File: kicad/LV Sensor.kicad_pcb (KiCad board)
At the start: 2 copper layers, 79.2 x 47 mm, 73 parts, among them IC1 MCP2517FDT-H_SL, IC2 L78L05ABUTR, IC3 TLV74133PDBVR, IC4 TLV74125PDBVR, IC5 MSPM0C1104SDGS20R, J1 Screw_Terminal_01x02, J16 USB_B_Micro, J2 Screw_Terminal_01x02, J3 Screw_Terminal_01x02, J4 Screw_Terminal_01x02, J5 Screw_Terminal_01x02, J6 43650-0401, SW1 SW_Push, U0 AP63205WU-7, U10 MCP3204-CI/P, U3 FT231XS-R, U6 DSC1001DL5-020.0000T, U7 ADS114S06BIPBSR, U8 LM2662MX/NOPB, U9 ATA6561-GAQW-N

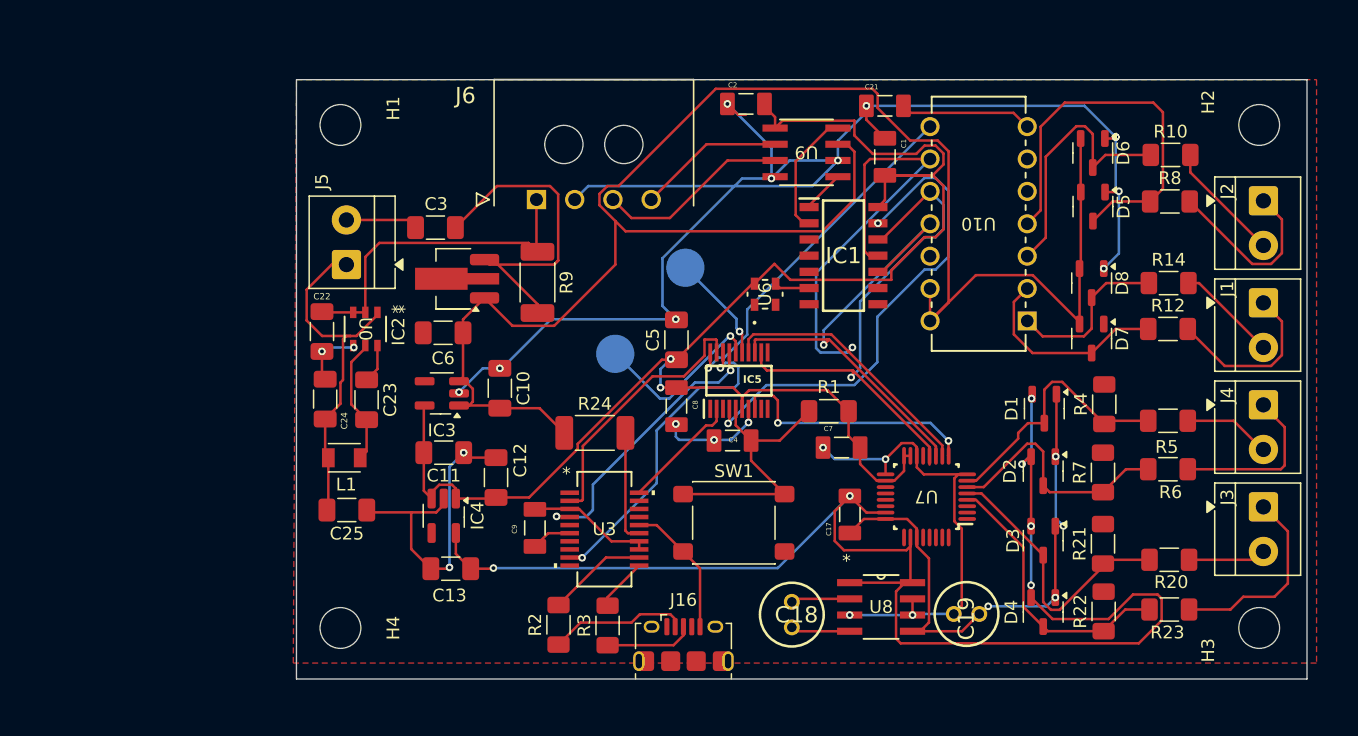
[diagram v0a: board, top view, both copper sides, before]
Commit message: finished v1
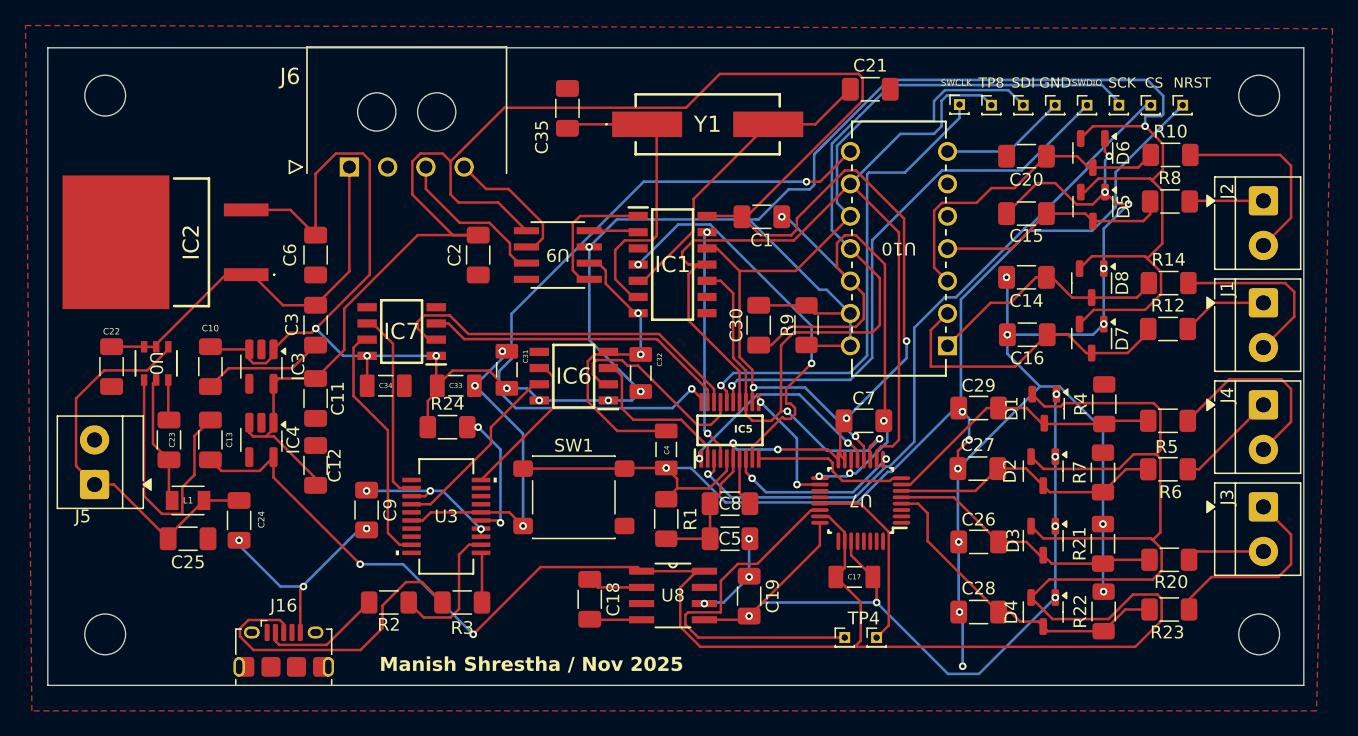
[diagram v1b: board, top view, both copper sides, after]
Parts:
- removed U6: DSC1001DL5-020.0000T, LV-Sensor-Footprints-Lib:CDFN4_2P5X2_MCH
- added C14: 0.1uF, Capacitor_SMD:C_1206_3216Metric_Pad1.33x1.80mm_HandSolder, F.Cu at (206.8, 67.8)
- added C15: 0.1uF, Capacitor_SMD:C_1206_3216Metric_Pad1.33x1.80mm_HandSolder, F.Cu at (206.8, 62.8)
- added C16: 0.1uF, Capacitor_SMD:C_1206_3216Metric_Pad1.33x1.80mm_HandSolder, F.Cu at (206.8, 72.2)
- added C20: 0.1uF, Capacitor_SMD:C_1206_3216Metric_Pad1.33x1.80mm_HandSolder, F.Cu at (206.8, 58.2)
- added C26: 0.1uF, Capacitor_SMD:C_1206_3216Metric_Pad1.33x1.80mm_HandSolder, F.Cu at (203.0, 88.5)
- added C27: 0.1uF, Capacitor_SMD:C_1206_3216Metric_Pad1.33x1.80mm_HandSolder, F.Cu at (202.9, 82.8)
- added C28: 0.1uF, Capacitor_SMD:C_1206_3216Metric_Pad1.33x1.80mm_HandSolder, F.Cu at (203.0, 94.0)
- added C29: 0.1uF, Capacitor_SMD:C_1206_3216Metric_Pad1.33x1.80mm_HandSolder, F.Cu at (203.0, 78.0)
- added C30: 0.1uF, Capacitor_SMD:C_1206_3216Metric_Pad1.33x1.80mm_HandSolder, F.Cu at (185.8, 71.5)
- added C31: 0.01uF, ADC2_AND_4:CAPC3216X140N, F.Cu at (166.0, 75.0)
- added C32: 0.01uF, ADC2_AND_4:CAPC3216X140N, F.Cu at (176.5, 75.2)
- added C33: 0.01uF, ADC2_AND_4:CAPC3216X140N, F.Cu at (162.0, 76.2)
- added C34: 0.01uF, ADC2_AND_4:CAPC3216X140N, F.Cu at (156.5, 76.2)
- added C35: 47pF, Capacitor_SMD:C_1206_3216Metric_Pad1.33x1.80mm_HandSolder, F.Cu at (170.8, 54.5)
- added IC6: ISO6721BDR, LV-Sensor-Footprints-Lib:SOIC127P600X175-8N, F.Cu at (171.2, 75.5)
- added IC7: ISO6721BDR, LV-Sensor-Footprints-Lib:SOIC127P600X175-8N, F.Cu at (157.8, 72.0)
- added TP10: TestPoint, Connector_PinHeader_1.00mm:PinHeader_1x01_P1.00mm_Vertical, F.Cu at (214.0, 54.2)
- added TP3: TestPoint, Connector_PinHeader_1.00mm:PinHeader_1x01_P1.00mm_Vertical, F.Cu at (192.5, 96.0)
- added TP4: TestPoint, Connector_PinHeader_1.00mm:PinHeader_1x01_P1.00mm_Vertical, F.Cu at (195.0, 96.0)
- added TP5: TestPoint, Connector_PinHeader_1.00mm:PinHeader_1x01_P1.00mm_Vertical, F.Cu at (209.0, 54.2)
- added TP6: TestPoint, Connector_PinHeader_1.00mm:PinHeader_1x01_P1.00mm_Vertical, F.Cu at (219.0, 54.2)
- added TP7: TestPoint, Connector_PinHeader_1.00mm:PinHeader_1x01_P1.00mm_Vertical, F.Cu at (216.5, 54.2)
- added TP8: TestPoint, Connector_PinHeader_1.00mm:PinHeader_1x01_P1.00mm_Vertical, F.Cu at (204.0, 54.2)
- added TP9: TestPoint, Connector_PinHeader_1.00mm:PinHeader_1x01_P1.00mm_Vertical, F.Cu at (206.5, 54.2)
- added Y1: 830017146, LV-Sensor-Footprints-Lib:830017146, F.Cu at (181.8, 55.8)
- C1, C2, C7: value 0.1µF -> 0.1uF; footprint ADC2_AND_4:CAPC3216X125N -> Capacitor_SMD:C_1206_3216Metric_Pad1.33x1.80mm_HandSolder
- C18, C19: footprint ADC2_AND_4:A750_5X7_ -> Capacitor_SMD:C_1206_3216Metric_Pad1.33x1.80mm_HandSolder
- C21: value 0.01µf -> 47pF; footprint ADC2_AND_4:CAPC3216X140N -> Capacitor_SMD:C_1206_3216Metric_Pad1.33x1.80mm_HandSolder
- C23: value 100nF -> 0.1uF
- C4: value 0.01 µF -> 0.01 uF
- C5: value 10u -> 10uF
- C8: value 100n -> 0.1uF; footprint ADC2_AND_4:CAPC3216X125N -> Capacitor_SMD:C_1206_3216Metric_Pad1.33x1.80mm_HandSolder
- C9: value 100nF -> 0.1uF; footprint ADC2_AND_4:CAPC3216X125N -> Capacitor_SMD:C_1206_3216Metric_Pad1.33x1.80mm_HandSolder
- IC2: value L78L05ABUTR -> MC7805CD2TR4G; footprint Package_TO_SOT_SMD:SOT-89-3_Handsoldering -> LV-Sensor-Footprints-Lib:MC7805CD2TR4G
- R24: footprint Resistor_SMD:R_2010_5025Metric_Pad1.40x2.65mm_HandSolder -> Resistor_SMD:R_1206_3216Metric_Pad1.30x1.75mm_HandSolder
- R9: value 1k -> 20k; footprint Resistor_SMD:R_2010_5025Metric_Pad1.40x2.65mm_HandSolder -> Resistor_SMD:R_1206_3216Metric_Pad1.30x1.75mm_HandSolder
- TP1, TP2: footprint TestPoint:TestPoint_Pad_D3.0mm -> Connector_PinHeader_1.00mm:PinHeader_1x01_P1.00mm_Vertical; moved to F.Cu
- moved TP2 34.0 mm to (211.5, 54.2), turned to 0 degrees
- moved TP1 33.3 mm to (201.5, 54.2), turned to 0 degrees
- moved J16 31.4 mm to (148.5, 97.0)
- moved J5 26.2 mm to (133.7, 84.0)
- moved C2 24.1 mm to (163.8, 66.0), turned to 90 degrees
- moved C10 22.8 mm to (142.8, 74.8), turned to 90 degrees
- moved IC2 22.5 mm to (139.5, 65.0), turned to 90 degrees
- moved C13 21.4 mm to (142.8, 80.5), turned to 90 degrees
- moved R9 21.4 mm to (189.5, 71.5)
- moved U9 21.1 mm to (170.0, 66.0)
- moved H1 18.6 mm to (134.5, 53.5)
- moved H4 18.5 mm to (134.5, 95.8)
- moved C19 17.1 mm to (185.0, 92.8), turned to -90 degrees
- moved C22 16.7 mm to (135.0, 74.8)
- moved U0 16.6 mm to (138.5, 74.5)
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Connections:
- net Net-(IC1-SCK) renamed SCK
- net Net-(IC1-SDI) renamed SDO
- net Net-(IC1-SDO) renamed SDI
- net Net-(IC5-PA1_/_NRST) renamed NRST
- C19 pad 1: -2V5 -> GND
- C19 pad 2: GND -> -2V5
- C21 pad 1: GND -> Net-(IC1-OSC2)
- C21 pad 2: Net-(U10-DGND) -> GND
- C3 pad 2: Net-(IC2-VIN) -> +12V
- C6 pad 1: GND -> +5V
- C6 pad 2: +5V -> GND
- IC1 pad 4: unconnected-(IC1-~{INT}-Pad4) -> CAN_FD_INT
- IC1 pad 5: unconnected-(IC1-OSC2-Pad5) -> Net-(IC1-OSC2)
- IC2 pad 1: +5V -> +12V
- IC2 pad 3: Net-(IC2-VIN) -> +5V
- IC5 pad 1: unconnected-(IC5-PA26_/_A1-Pad1) -> ADC_DRDY
- IC5 pad 10: unconnected-(IC5-PA6-Pad10) -> ADC_START
- IC5 pad 11: unconnected-(IC5-PA11-Pad11) -> ADC_RESET
- IC5 pad 3: unconnected-(IC5-PA28_/_A5-Pad3) -> EXTERNAL_CS
- IC5 pad 9: unconnected-(IC5-PA4-Pad9) -> CAN_FD_INT
- R9 pad 1: +12V -> +5V
- R9 pad 2: Net-(IC2-VIN) -> +5V
- U10 pad 7: Net-(U10-DGND) -> GND
- U3 pad 2: UART0_RTS -> UART0_RTS_ISOLA
- U3 pad 20: UART0_TX -> UART0_TX_ISOLA
- U3 pad 4: UART0_RX -> UART0_RX_ISOLA
- U3 pad 9: UART0_CTS -> UART0_CTS_ISOLA
- U7 pad 13: unconnected-(U7-DRDY_N-Pad13) -> ADC_DRDY
- U7 pad 18: +3V3 -> ADC_RESET
- U7 pad 21: unconnected-(U7-GPIO1-Pad21) -> Net-(U7-GPIO1)
- U7 pad 22: unconnected-(U7-GPIO0-Pad22) -> Net-(U7-GPIO0)
- U7 pad 8: GND -> ADC_START
- U8 pad 7: GND -> unconnected-(U8-OSC-Pad7)
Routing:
- net +5V: track 144.0 -> 213.0 mm, vias 0 -> 9
- net +2V5: track 116.4 -> 175.7 mm, vias 6 -> 2
- net NRST: track 21.7 -> 80.7 mm, vias 0 -> 1
- net EXTERNAL_CS: track 0.00 -> 55.9 mm, vias 0 -> 1
- net GND: track 212.0 -> 262.6 mm, vias 22 -> 30
- net SCK: track 38.6 -> 81.8 mm, vias 1 -> 2
- net +3V3: track 126.5 -> 169.7 mm, vias 2 -> 4
- net Net-(IC5-PA19_/_SWDIO): track 8.48 -> 43.7 mm
- net CAN_FD_INT: track 0.00 -> 31.9 mm, vias 0 -> 2
- net Net-(U7-GPIO0): track 0.00 -> 29.1 mm
- net CS_ADC4: track 27.7 -> 56.0 mm, vias 1 -> 2
- net Net-(IC2-VIN): track 27.6 -> 0.00 mm
- net Net-(IC1-OSC2): track 0.00 -> 24.3 mm
- net Net-(IC5-PA20_/_A6_/_SWCLK): track 14.1 -> 38.4 mm
- net Net-(IC1-OSC1): track 2.77 -> 23.8 mm
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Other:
- board size 79.2 x 47 mm -> 98.5 x 50 mm
- board text added: "CS"
- board text added: "GND"
- board text added: "Manish Shrestha / Nov 2025"
- board text added: "NRST"
- board text added: "SCK"
- board text added: "SDI"
- board text added: "SWCLK"
- board text added: "SWDIO"
- board text removed: "- Manish Shrestha / Nov 2025"
